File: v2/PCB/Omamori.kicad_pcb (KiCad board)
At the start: 2 copper layers, 26 x 36 mm, 12 parts, among them U1 BQ25504, U2 ATtiny13A-SSU

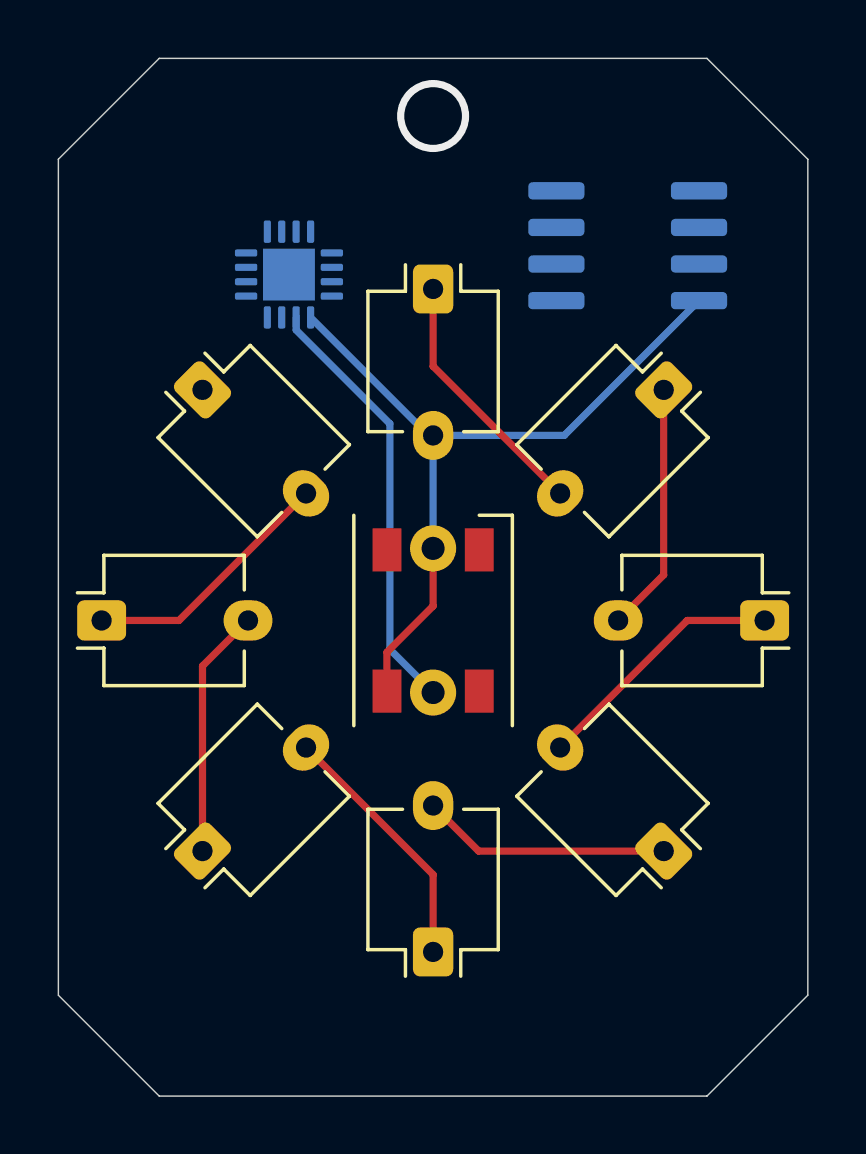
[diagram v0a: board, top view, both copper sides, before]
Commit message: Modified PCB and updated Software.
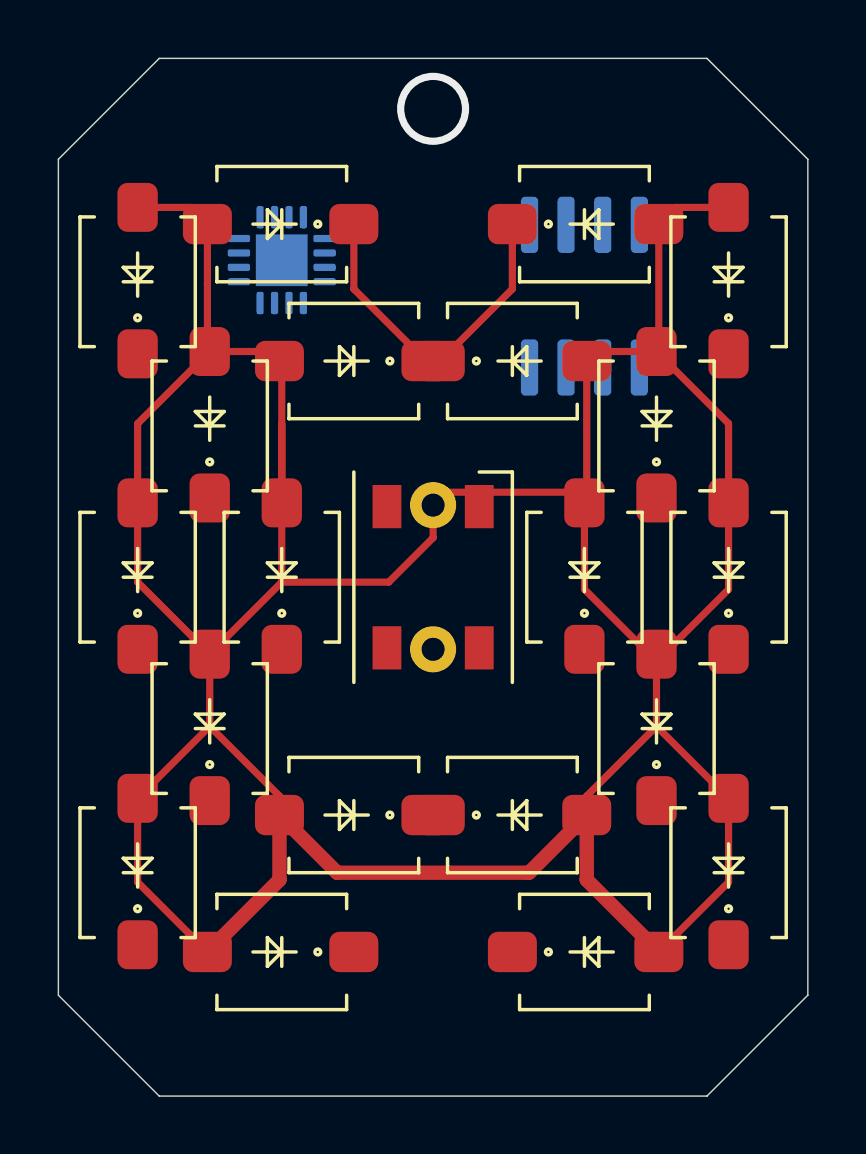
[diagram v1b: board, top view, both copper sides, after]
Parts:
- added D10: BPW34, own_footprints:Osram_DIL2_4.3x4.65mm_P5.08mm, F.Cu at (180.2, 91.0)
- added D11: BPW34, own_footprints:Osram_DIL2_4.3x4.65mm_P5.08mm, F.Cu at (190.2, 90.8)
- added D12: BPW34, own_footprints:Osram_DIL2_4.3x4.65mm_P5.08mm, F.Cu at (179.8, 106.8)
- added D13: BPW34, own_footprints:Osram_DIL2_4.3x4.65mm_P5.08mm, F.Cu at (187.8, 95.8)
- added D14: BPW34, own_footprints:Osram_DIL2_4.3x4.65mm_P5.08mm, F.Cu at (169.8, 111.2)
- added D15: BPW34, own_footprints:Osram_DIL2_4.3x4.65mm_P5.08mm, F.Cu at (187.8, 106.2)
- added D16: BPW34, own_footprints:Osram_DIL2_4.3x4.65mm_P5.08mm, F.Cu at (172.2, 106.2)
- added D17: BPW34, own_footprints:Osram_DIL2_4.3x4.65mm_P5.08mm, F.Cu at (177.2, 111.5)
- added D18: BPW34, own_footprints:Osram_DIL2_4.3x4.65mm_P5.08mm, F.Cu at (179.8, 91.0)
- added D19: BPW34, own_footprints:Osram_DIL2_4.3x4.65mm_P5.08mm, F.Cu at (172.2, 95.8)
- added D20: BPW34, own_footprints:Osram_DIL2_4.3x4.65mm_P5.08mm, F.Cu at (177.2, 86.2)
- added D21: BPW34, own_footprints:Osram_DIL2_4.3x4.65mm_P5.08mm, F.Cu at (182.8, 86.2)
- CSuper1: footprint Capacitor_THT:C_Rect_L7.2mm_W2.5mm_P5.00mm_FKS2_FKP2_MKS2_MKP2 -> Capacitor_THT:C_Radial_D10.0mm_H12.5mm_P5.00mm
- D1, D2, D3, D4, D5, D6, D7, D8: footprint OptoDevice:Osram_DIL2_4.3x4.65mm_P5.08mm -> own_footprints:Osram_DIL2_4.3x4.65mm_P5.08mm
- D9: footprint LED_SMD:LED_WS2812B_PLCC4_5.0x5.0mm_P3.2mm -> LED_SMD:LED_SK6812_PLCC4_5.0x5.0mm_P3.2mm
- moved D8 23.2 mm to (182.8, 111.5), turned to 0 degrees
- moved D6 11.3 mm to (190.2, 111.2), turned to 90 degrees
- moved D7 9.28 mm to (190.2, 101.0), turned to 90 degrees
- moved D3 7.52 mm to (174.8, 101.0), turned to 90 degrees
- moved D5 7.52 mm to (185.2, 101.0), turned to 90 degrees
- moved D4 4.76 mm to (180.2, 106.8), turned to 0 degrees
- moved D1 2.57 mm to (169.8, 90.8), turned to 90 degrees
- moved U2 2.30 mm to (185.2, 88.8), turned to 270 degrees
- moved D2 1.60 mm to (169.8, 101.0), turned to 90 degrees
- moved CSuper1 1.50 mm to (180.0, 101.0)
- moved D9 1.50 mm to (180.0, 98.5)
- moved U1 0.56 mm to (174.8, 87.5)
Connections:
- D1 pad 2: Net-(D1-Pad2) -> GND
- D2 pad 1: Net-(D1-Pad2) -> Net-(D1-Pad1)
- D2 pad 2: Net-(D2-Pad2) -> GND
- D3 pad 1: Net-(D2-Pad2) -> Net-(D1-Pad1)
- D3 pad 2: Net-(D3-Pad2) -> GND
- D4 pad 1: Net-(D3-Pad2) -> Net-(D1-Pad1)
- D4 pad 2: Net-(D4-Pad2) -> GND
- D5 pad 1: Net-(D4-Pad2) -> Net-(D1-Pad1)
- D5 pad 2: Net-(D5-Pad2) -> GND
- D6 pad 1: Net-(D5-Pad2) -> Net-(D1-Pad1)
- D6 pad 2: Net-(D6-Pad2) -> GND
- D7 pad 1: Net-(D6-Pad2) -> Net-(D1-Pad1)
- D7 pad 2: Net-(D7-Pad2) -> GND
- D8 pad 1: Net-(D7-Pad2) -> Net-(D1-Pad1)
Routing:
- net GND: track 26.7 -> 140.2 mm
- net Net-(CSuper1-Pad1): track 15.0 -> 0.00 mm
- net Net-(D1-Pad1): track 0.00 -> 11.6 mm
- net Net-(D5-Pad2): track 8.92 -> 0.00 mm
- net Net-(D1-Pad2): track 8.92 -> 0.00 mm
- net Net-(D7-Pad2): track 8.92 -> 0.00 mm
- net Net-(D3-Pad2): track 8.92 -> 0.00 mm
- net Net-(D6-Pad2): track 8.65 -> 0.00 mm
- net Net-(D2-Pad2): track 8.65 -> 0.00 mm
- net Net-(D4-Pad2): track 8.65 -> 0.00 mm
